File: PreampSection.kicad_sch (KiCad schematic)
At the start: 106 parts, among them Q1 TIP 50, T1 AS-05T240, U1 LR8, U2 LT1085-ADJ

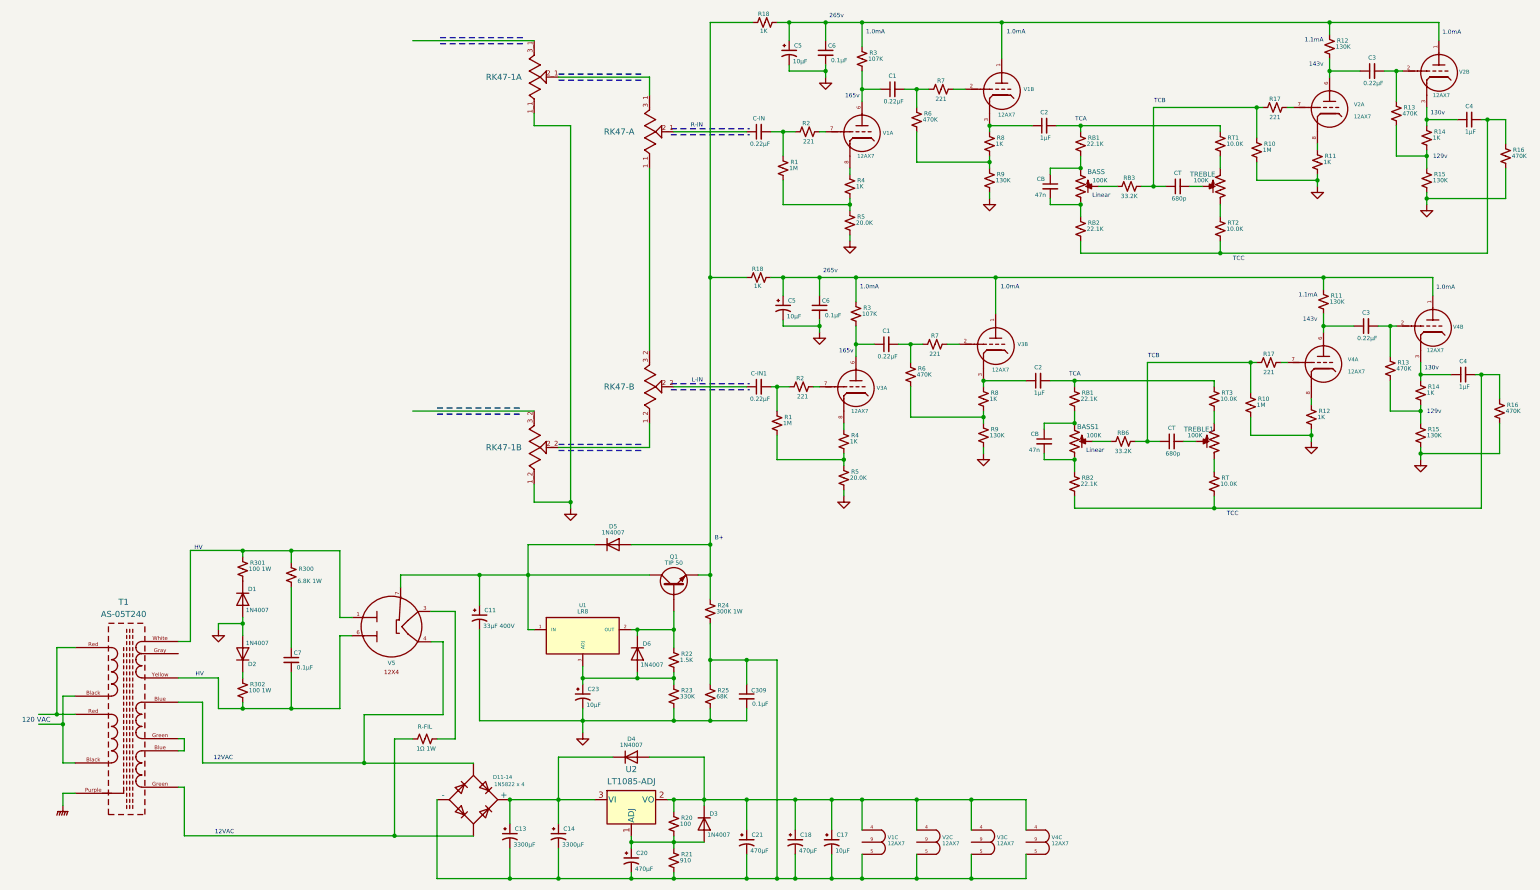
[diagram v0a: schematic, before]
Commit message: Completed Schematics :
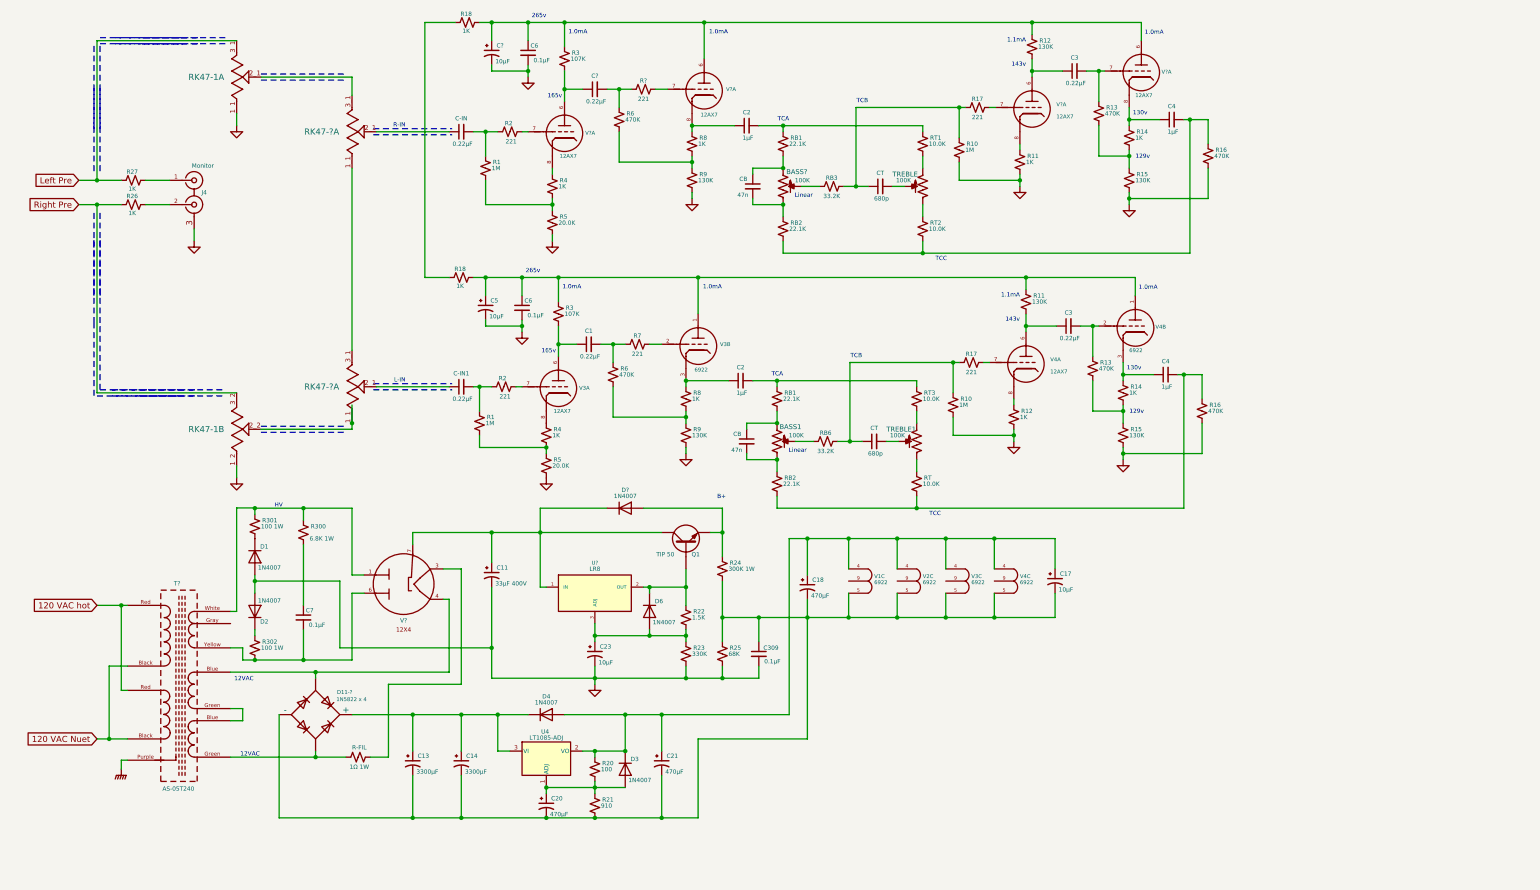
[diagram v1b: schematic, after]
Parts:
- removed BASS: 100K, symbol Resistors:R_Potentiometer_US
- removed C1 (x2), C3 (x2): 0.22µF, symbol Device:C_Small
- removed C2 (x2), C4 (x2): 1µF, symbol Device:C_Small
- removed C5 (x2): 10µF, symbol Device:C_Polarized_Small_US
- removed C6 (x2): 0.1µF, symbol Device:C_Small
- removed CB (x2): 47n, symbol Device:C_Small
- removed CT (x2): 680p, symbol Device:C_Small
- removed D11-14: 1N5822 x 4, Diode_THT:Diode_Bridge_GeneSiC_KBPC_W, symbol Diode_Bridge:KBPC1501W
- removed D5: 1N4007, Diode_THT:D_DO-41_SOD81_P10.16mm_Horizontal, symbol Diode:1N4007
- removed R1 (x2), R10 (x2): 1M, symbol Resistors:R_Small_US
- removed R11, R12, R14 (x2), R18 (x2), R4 (x2), R8 (x2): 1K, symbol Resistors:R_Small_US
- removed R11, R12, R15 (x2), R9 (x2): 130K, symbol Resistors:R_Small_US
- removed R13 (x2), R16 (x2), R6 (x2): 470K, symbol Resistors:R_Small_US
- removed R17 (x2), R2 (x2), R7 (x2): 221, symbol Resistors:R_Small_US
- removed R3 (x2): 107K, symbol Resistors:R_Small_US
- removed R5 (x2): 20.0K, symbol Resistors:R_Small_US
- removed RB1 (x2), RB2 (x2): 22.1K, symbol Resistors:R_Small_US
- removed RK47-: RK47-A, RK27112A0S20C0A103:TRIM_RK27112A0S20C0A103, symbol RK27112A0S20C0A103:RK27112A0S20C0A103
- removed T1: AS-05T240, symbol My_Transformers:AS-05T240
- removed U1: LR8, Package_TO_SOT_THT:TO-92_Inline, symbol Regulator_Linear:LR8N3-G
- removed U2: LT1085-ADJ, symbol Regulator_Linear:LT1085-ADJ
- removed unit 1 of V1
- removed unit 2 of V1
- removed unit 1 of V2
- removed unit 2 of V2
- removed V5: ~, symbol My Tubes:12X4
- added BASS?: 100K, symbol Resistors:R_Potentiometer_US
- added C1, C3 (x2), C?: 0.22µF, symbol Device:C_Small
- added C2 (x2), C4 (x2): 1µF, symbol Device:C_Small
- added C5, C?: 10µF, symbol Device:C_Polarized_Small_US
- added C6 (x2): 0.1µF, symbol Device:C_Small
- added CB (x2): 47n, symbol Device:C_Small
- added CT (x2): 680p, symbol Device:C_Small
- added D11-?: 1N5822 x 4, Diode_THT:Diode_Bridge_GeneSiC_KBPC_W, symbol Diode_Bridge:KBPC1501W
- added D?: 1N4007, Diode_THT:D_DO-41_SOD81_P10.16mm_Horizontal, symbol Diode:1N4007
- added J4: Monitor, symbol Connector:Conn_Coaxial_x2
- added R1 (x2), R10 (x2): 1M, symbol Resistors:R_Small_US
- added R11, R12, R14 (x2), R18 (x2), R26, R27, R4 (x2), R8 (x2): 1K, symbol Resistors:R_Small_US
- added R11, R12, R15 (x2), R9 (x2): 130K, symbol Resistors:R_Small_US
- added R13 (x2), R16 (x2), R6 (x2): 470K, symbol Resistors:R_Small_US
- added R17 (x2), R2 (x2), R7, R?: 221, symbol Resistors:R_Small_US
- added R3 (x2): 107K, symbol Resistors:R_Small_US
- added R5 (x2): 20.0K, symbol Resistors:R_Small_US
- added RB1 (x2), RB2 (x2): 22.1K, symbol Resistors:R_Small_US
- added RK47-? (x2): RK47-A, RK27112A0S20C0A103:TRIM_RK27112A0S20C0A103, symbol RK27112A0S20C0A103:RK27112A0S20C0A103
- added T?: AS-05T240, symbol My_Transformers:AS-05T240
- added U4: LT1085-ADJ, symbol Regulator_Linear:LT1085-ADJ
- added U?: LR8, Package_TO_SOT_THT:TO-92_Inline, symbol Regulator_Linear:LR8N3-G
- added V? (x4): 12AX7, symbol My Tubes:12AX7
- added V?: ~, symbol My Tubes:12X4
- V1, V2, V3, V4: value 12AX7 -> 6922
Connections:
- net GND: now also C5.2, C6.2, C6.2, C?.2, J4.3 (EXT), R10.2, R10.2, R11.2, R12.2, R15.2, R15.2, R16.2, R16.2, R5.2, R5.2, R9.2, R9.2
- net GNDPWR: now also T?.Purple (AB)
- net at C17.1, C18.1, C21.1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: now also U4.2 (VO)
- net at C13.2, C14.2, C17.2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: now also D11-?. (+)
- net at RK47-1.2_2: now also RK47-?.1_1
- net Right Pre: now reaches RK47-1.3_2
- net Right Pre: now also R26.1
- net at RB3.2: now also CT.1, R10.1, R17.1
- net at TREBLE. (2): now also CT.2
- net at C-IN.1: now also RK47-?.2_1
- net at RK47-1.2_1: now also RK47-?.3_1
- net at D6.1 (K), Q1.2, R22.1: now also U?.2 (OUT)
- net at C23.1, D6.2 (A), R22.2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: now also U?.3 (ADJ)
- net at V3.6: now also C1.1, R3.2
- net at C11.1, Q1.1: now also D?.1 (K), U?.1 (IN), V?.7
- net at Q1.3, R24.1: now also D?.2 (A)
- net at RB3.1: now also BASS?. (2)
- net at C20.1, D3.2 (A), R20.2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: now also U4.1 (ADJ)
- net at C13.1, C14.1, D4.1 (K): now also D11-?. (+), U4.3 (VI)
- net at V3.1, V4.1: now also C5.1, C6.1, R11.1, R18.2, R3.1
- net at R-FIL.1: now also D11-?. (+), T?.Green (OUT2B)
- net at BASS1. (2): now also CB.2, RB2.1
- net at C-IN1.2: now also R1.1, R2.1
- net at V3.7: now also R2.2
- net at RB6.2: now also CT.1, R10.1, R17.1
- net at C-IN.2: now also R1.1, R2.1
- net at RT2.2: now also C4.2, R16.1, RB2.2
- net at RT.2: now also C4.2, R16.1, RB2.2
- net at RT1.1: now also C2.2, RB1.1
- net at V3.2: now also R7.2
- net at R300.1, R301.1: now also T?.White (OUT1A), V?.1
- net at C7.2, R302.2: now also T?.Yellow (OUT1B), V?.6
- net at C-IN1.1: now also RK47-?.2_1
- net at V4.8: now also R12.1
- net at V3.3: now also C2.1, R8.1
- net at R-FIL.2: now also V?.3
- net at V4.2: now also C3.2, R13.1
- net at V4.3: now also C4.1, R14.1
- net at V4.6: now also C3.1, R11.2
- net at RT3.1: now also C2.2, RB1.1
- net at V4.7: now also R17.2
- net at TREBLE1. (2): now also CT.2
- net at V3.8: now also R4.1
- net Left Pre: now reaches RK47-1.3_1
- net Left Pre: now also R27.1
- new net: C6.1, C?.1, R12.1, R18.2, R3.1, V?.6, V?.6
- new net: C?.1, R3.2, V?.6
- new net: J4.1 (IN1), R27.2
- new net: J4.2 (IN2), R26.2
- new net: D11-?. (+), T?.Blue (OUT2A), V?.4
- new net: C3.2, R13.1, V?.7
- new net: R13.2, R14.2, R15.1 (x2)
- new net: R1.2, R4.2, R5.1 (x2)
- new net: R11.1, V?.8
- new net: RK47-?.1_1, RK47-?.3_1
- new net: C?.2, R6.1, R?.1
- new net: R6.2, R8.2, R9.1 (x2)
- new net: C1.2, R6.1, R7.1
- new net: C3.1, R12.2, V?.6
- new net: C2.1, R8.1, V?.8
- new net: R18.1, R18.1
- new net: BASS?. (2), CB.2, RB2.1
- new net: R?.2, V?.7
- new net: R2.2, V?.7
- new net: BASS1. (2), CB.1, RB1.2
- new net: R4.1, V?.8
- new net: BASS?. (2), CB.1, RB1.2
- new net: C4.1, R14.1, V?.8
- new net: R17.2, V?.7
- new net: T?.Blue (OUT2A), T?.Green (OUT2B)
- new net 120 VAC Nuet: T?.Black (AB)
- new net 120 VAC hot: T?.Red (AA)
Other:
- note removed: "120 VAC"
